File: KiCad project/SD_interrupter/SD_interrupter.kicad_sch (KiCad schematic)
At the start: 38 parts, among them J1 Micro_SD_Card_Det, J2 AVR-ISP-6, J3 DIN-5, J4 Jack-DC, J5 VCC, SW1 BL_SW, SW2 MAIN_SW, SW3 UP_SW, SW4 DN_SW, SW5 OK_SW, U1 LM7805_TO220, U2 4050, U3 AMS1117-3.3, U4 ATmega168-20P, U5 4N25, U6 IFE91A, Y1 Crystal

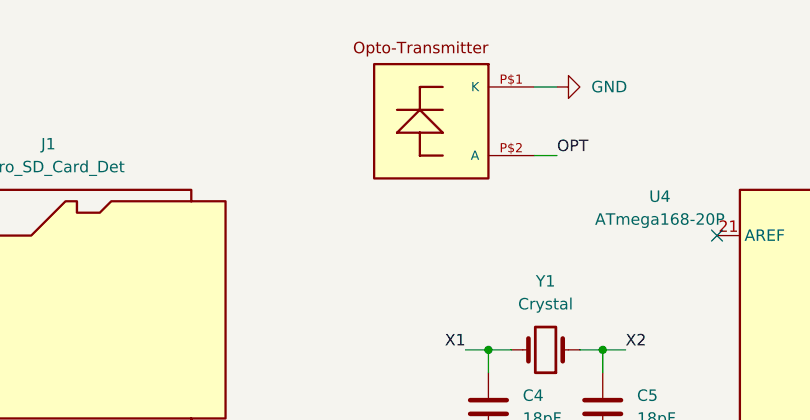
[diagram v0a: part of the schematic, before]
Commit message: safety switch
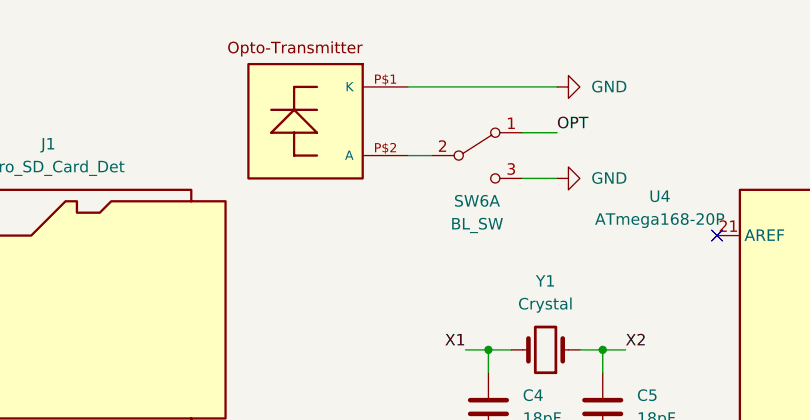
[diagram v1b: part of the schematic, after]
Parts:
- added SW6: BL_SW, Switch:Switch 12x6mm, symbol Switch:SW_DPDT_x2
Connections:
- net GND: now also SW6.3 (C)
- net OPT: now also SW6.1 (A); no longer U6.P$2 (A)
- new net: SW6.2 (B), U6.P$2 (A)
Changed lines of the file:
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@@
+    (stroke (width 0) (type default) (color 0 0 0 0))
+  )
+  (wire (pts (xy 193.04 33.02) (xy 195.58 33.02))
     (stroke (width 0) (type default) (color 0 0 0 0))
   )
@@
     (stroke (width 0) (type default) (color 0 0 0 0))
   )
-  (wire (pts (xy 207.01 25.4) (xy 209.55 25.4))
+  (wire (pts (xy 193.04 25.4) (xy 209.55 25.4))
     (stroke (width 0) (type default) (color 0 0 0 0))
   )
@@
     (stroke (width 0) (type default) (color 0 0 0 0))
   )
+  (wire (pts (xy 205.74 30.48) (xy 209.55 30.48))
+    (stroke (width 0) (type default) (color 0 0 0 0))
+  )
   (wire (pts (xy 41.91 114.3) (xy 43.18 114.3))
     (stroke (width 0) (type default) (color 0 0 0 0))
@@
     (stroke (width 0) (type default) (color 0 0 0 0))
   )
+  (wire (pts (xy 205.74 35.56) (xy 209.55 35.56))
+    (stroke (width 0) (type default) (color 0 0 0 0))
+  )
   (wire (pts (xy 257.81 52.07) (xy 259.08 52.07))
     (stroke (width 0) (type default) (color 0 0 0 0))
@@
     (stroke (width 0) (type default) (color 0 0 0 0))
   )
-  (wire (pts (xy 207.01 33.02) (xy 209.55 33.02))
-    (stroke (width 0) (type default) (color 0 0 0 0))
-  )
   (wire (pts (xy 71.12 121.92) (xy 71.12 123.19))
     (stroke (width 0) (type default) (color 0 0 0 0))
@@
     (effects (font (size 1.27 1.27)) (justify left bottom))
   )
-  (label "OPT" (at 209.55 33.02 0)
+  (label "OPT" (at 209.55 30.48 0)
     (effects (font (size 1.27 1.27)) (justify left bottom))
   )
@@
     (pin "1")
   )
+  (symbol (lib_id "power:GND") (at 209.55 35.56 90) (unit 1)
+    (in_bom yes) (on_board yes) (fields_autoplaced)
+    (property "Reference" "#PWR05" (id 0) (at 215.9 35.56 0)
+      (effects (font (size 1.27 1.27)) hide)
+    )
+    (property "Value" "GND" (id 1) (at 213.36 35.5599 90)
+      (effects (font (size 1.27 1.27)) (justify right))
+    )
+    (property "Footprint" "" (id 2) (at 209.55 35.56 0)
+      (effects (font (size 1.27 1.27)) hide)
+    )
+    (property "Datasheet" "" (id 3) (at 209.55 35.56 0)
+      (effects (font (size 1.27 1.27)) hide)
+    )
+    (pin "1")
+  )
   (symbol (lib_id "power:GND") (at 209.55 25.4 90) (unit 1)
     (in_bom yes) (on_board yes) (fields_autoplaced)
@@
     (pin "1")
   )
+  (symbol (lib_id "Switch:SW_DPDT_x2") (at 200.66 33.02 0) (unit 1)
+    (in_bom yes) (on_board yes)
+    (property "Reference" "SW6" (id 0) (at 200.66 38.1 0))
+    (property "Value" "BL_SW" (id 1) (at 200.66 40.64 0))
+    (property "Footprint" "Switch:Switch 12x6mm" (id 2) (at 200.66 33.02 0)
+      (effects (font (size 1.27 1.27)) hide)
+    )
+    (property "Datasheet" "~" (id 3) (at 200.66 33.02 0)
+      (effects (font (size 1.27 1.27)) hide)
+    )
+    (pin "1")
+    (pin "2")
+    (pin "3")
+    (pin "4")
+    (pin "5")
+    (pin "6")
+  )
   (symbol (lib_id "power:PWR_FLAG") (at 43.18 24.13 0) (unit 1)
     (in_bom yes) (on_board yes) (fields_autoplaced)
@@
     (pin "8")
   )
-  (symbol (lib_id "IFE91A:IFE91A") (at 194.31 27.94 180) (unit 1)
-    (in_bom yes) (on_board yes) (fields_autoplaced)
-    (property "Reference" "U6" (id 0) (at 194.31 27.94 0)
+  (symbol (lib_id "IFE91A:IFE91A") (at 180.34 27.94 180) (unit 1)
+    (in_bom yes) (on_board yes) (fields_autoplaced)
+    (property "Reference" "U6" (id 0) (at 180.34 27.94 0)
       (effects (font (size 1.27 1.27)) (justify left bottom) hide)
     )
-    (property "Value" "IFE91A" (id 1) (at 194.31 27.94 0)
+    (property "Value" "IFE91A" (id 1) (at 180.34 27.94 0)
       (effects (font (size 1.27 1.27)) (justify left bottom) hide)
     )
-    (property "Footprint" "IFE91A:OPTO-TRANSMITTER" (id 2) (at 194.31 27.94 0)
+    (property "Footprint" "IFE91A:OPTO-TRANSMITTER" (id 2) (at 180.34 27.94 0)
       (effects (font (size 1.27 1.27)) (justify left bottom) hide)
     )
-    (property "Datasheet" "" (id 3) (at 194.31 27.94 0)
+    (property "Datasheet" "" (id 3) (at 180.34 27.94 0)
       (effects (font (size 1.27 1.27)) (justify left bottom) hide)
     )
@@
       (reference "#PWR04") (unit 1) (value "GND") (footprint "")
     )
+    (path "/620a2a80-1907-4e37-b42f-7d6530a57325"
+      (reference "#PWR05") (unit 1) (value "GND") (footprint "")
+    )
     (path "/f5ad944c-d4c5-448f-becd-1e591c8b8925"
       (reference "#PWR0101") (unit 1) (value "GND") (footprint "")
@@
       (reference "SW5") (unit 1) (value "OK_SW") (footprint "Button_Switch_THT:SW_PUSH_6mm_H7.3mm")
     )
+    (path "/7b12841d-819a-4272-a88b-3981c7c9c889"
+      (reference "SW6") (unit 1) (value "BL_SW") (footprint "Switch:Switch 12x6mm")
+    )
     (path "/fa495c25-f5e1-4425-ae98-e5a137fd7f85"
